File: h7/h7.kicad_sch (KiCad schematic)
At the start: 0 parts

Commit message: updated pinout
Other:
- added sheet mcu (mcu.kicad_sch)
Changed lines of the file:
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@@
 	(generator_version "9.0")
 	(paper "A4")
+	(sheet
+		(at 31.115 20.955)
+		(size 17.78 10.16)
+		(exclude_from_sim no)
+		(in_bom yes)
+		(on_board yes)
+		(dnp no)
+		(fields_autoplaced yes)
+		(stroke
+			(width 0.1524)
+			(type solid)
+		)
+		(fill
+			(color 0 0 0 0.0000)
+		)
+		(property "Sheetname" "mcu"
+			(at 31.115 20.2434 0)
+			(effects
+				(font
+					(size 1.27 1.27)
+				)
+				(justify left bottom)
+			)
+		)
+		(property "Sheetfile" "mcu.kicad_sch"
+			(at 31.115 31.6996 0)
+			(effects
+				(font
+					(size 1.27 1.27)
+				)
+				(justify left top)
+			)
+		)
+		(instances
+			(project "h7"
+				(path "/521e8535-7092-4752-992a-adc9653ebbe6"
+					(page "2")
+				)
+			)
+		)
+	)
 	(sheet_instances
 		(path "/"

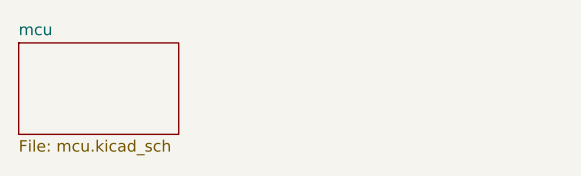
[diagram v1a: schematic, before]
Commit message: todays progress with schematic and pinout
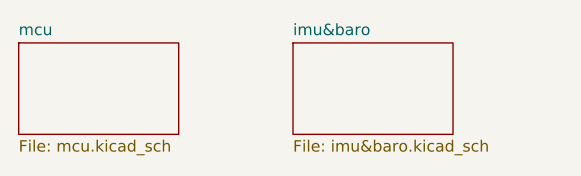
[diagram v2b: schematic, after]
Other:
- added sheet imu&baro (imu&baro.kicad_sch)
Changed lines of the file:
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@@
 	(paper "A4")
+	(sheet
+		(at 61.595 20.955)
+		(size 17.78 10.16)
+		(exclude_from_sim no)
+		(in_bom yes)
+		(on_board yes)
+		(dnp no)
+		(fields_autoplaced yes)
+		(stroke
+			(width 0.1524)
+			(type solid)
+		)
+		(fill
+			(color 0 0 0 0.0000)
+		)
+		(property "Sheetname" "imu&baro"
+			(at 61.595 20.2434 0)
+			(effects
+				(font
+					(size 1.27 1.27)
+				)
+				(justify left bottom)
+			)
+		)
+		(property "Sheetfile" "imu&baro.kicad_sch"
+			(at 61.595 31.6996 0)
+			(effects
+				(font
+					(size 1.27 1.27)
+				)
+				(justify left top)
+			)
+		)
+		(instances
+			(project "h7"
+				(path "/521e8535-7092-4752-992a-adc9653ebbe6"
+					(page "3")
+				)
+			)
+		)
+	)
 	(sheet
 		(at 31.115 20.955)
